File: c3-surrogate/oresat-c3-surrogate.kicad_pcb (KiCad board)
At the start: 2 copper layers, 99.8 x 94.6 mm, 61 parts, among them J1 J-SAMTEC-TFM-120-X1-XXX-D-RA, J2 Conn_01x04, J3 Terminal Block, J5 Header, J6 Header, Q1 PMV45EN, Q2 DMP3050LVT-7, Q3 PMV45EN, Q4 DMP3050LVT-7, SW1 Slide Switch, SW2 Slide Switch, U1 Trinket-M0, U2 Seeed-USB-to-UART, U3 MAX892LEUA+T

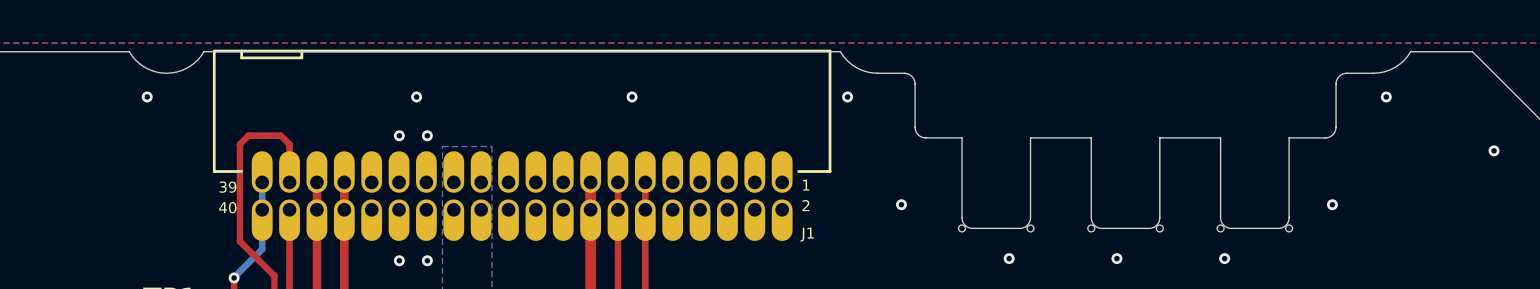
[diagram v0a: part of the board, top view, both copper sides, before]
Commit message: finished schematic, updated pcb
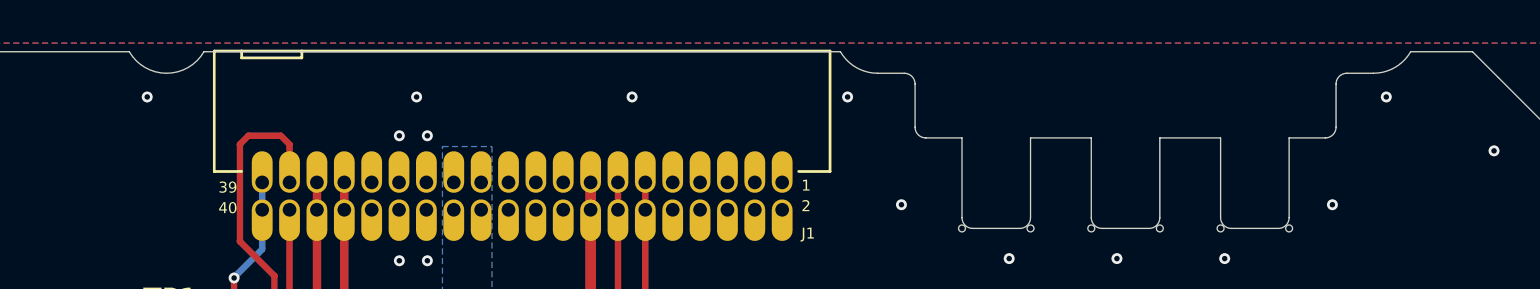
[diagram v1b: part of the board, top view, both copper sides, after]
